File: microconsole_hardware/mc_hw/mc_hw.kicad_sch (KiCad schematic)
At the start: 39 parts, among them SW1 DPAD - UP, SW10 START, SW11 L1, SW12 R1, SW13 L2, SW14 R2, SW16 Joystick, SW17 Joystick, SW2 DPAD - DOWN, SW3 DPAD - LEFT, SW4 DPAD - RIGHT, SW5 A, SW6 B, SW7 X, SW8 Y, SW9 SELECT, U1 ILI9341 / ST7796S SPI LCD, U2 MAX98357A, U3 MCP23017x-x-SO

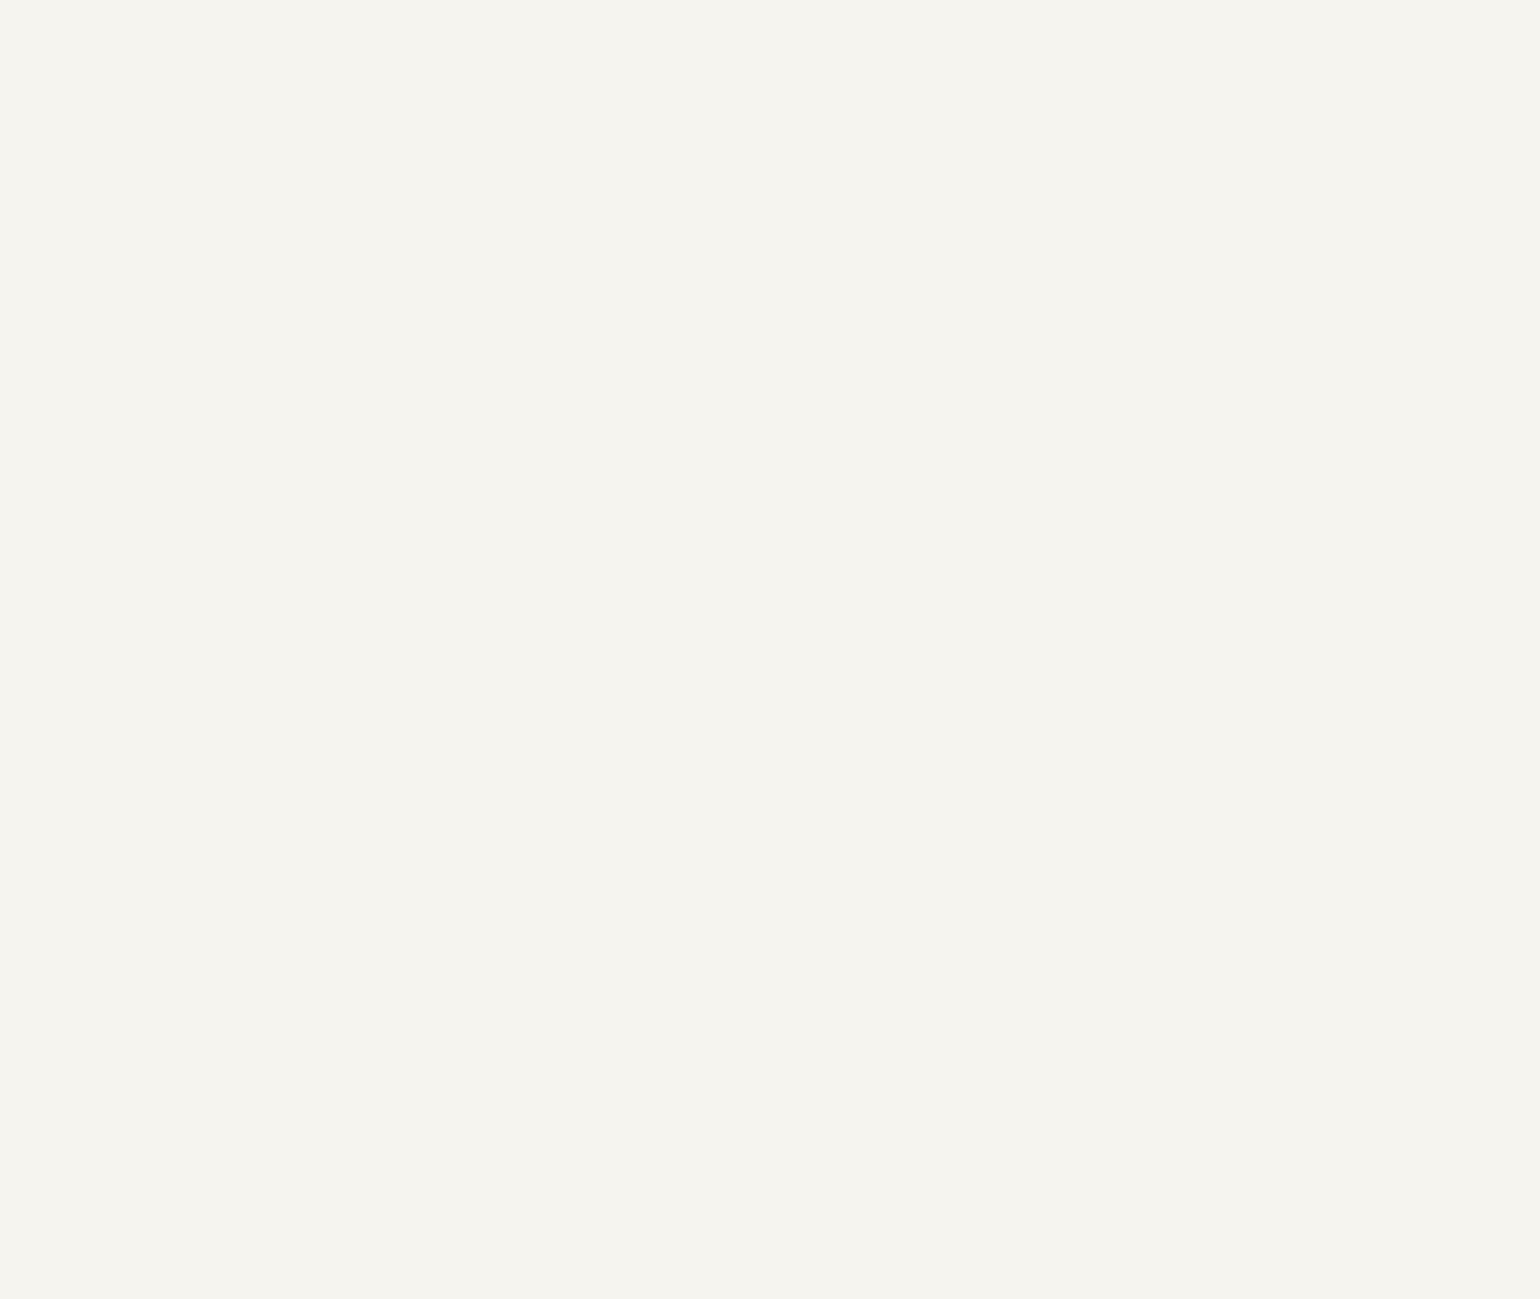
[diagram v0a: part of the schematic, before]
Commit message: hardware update
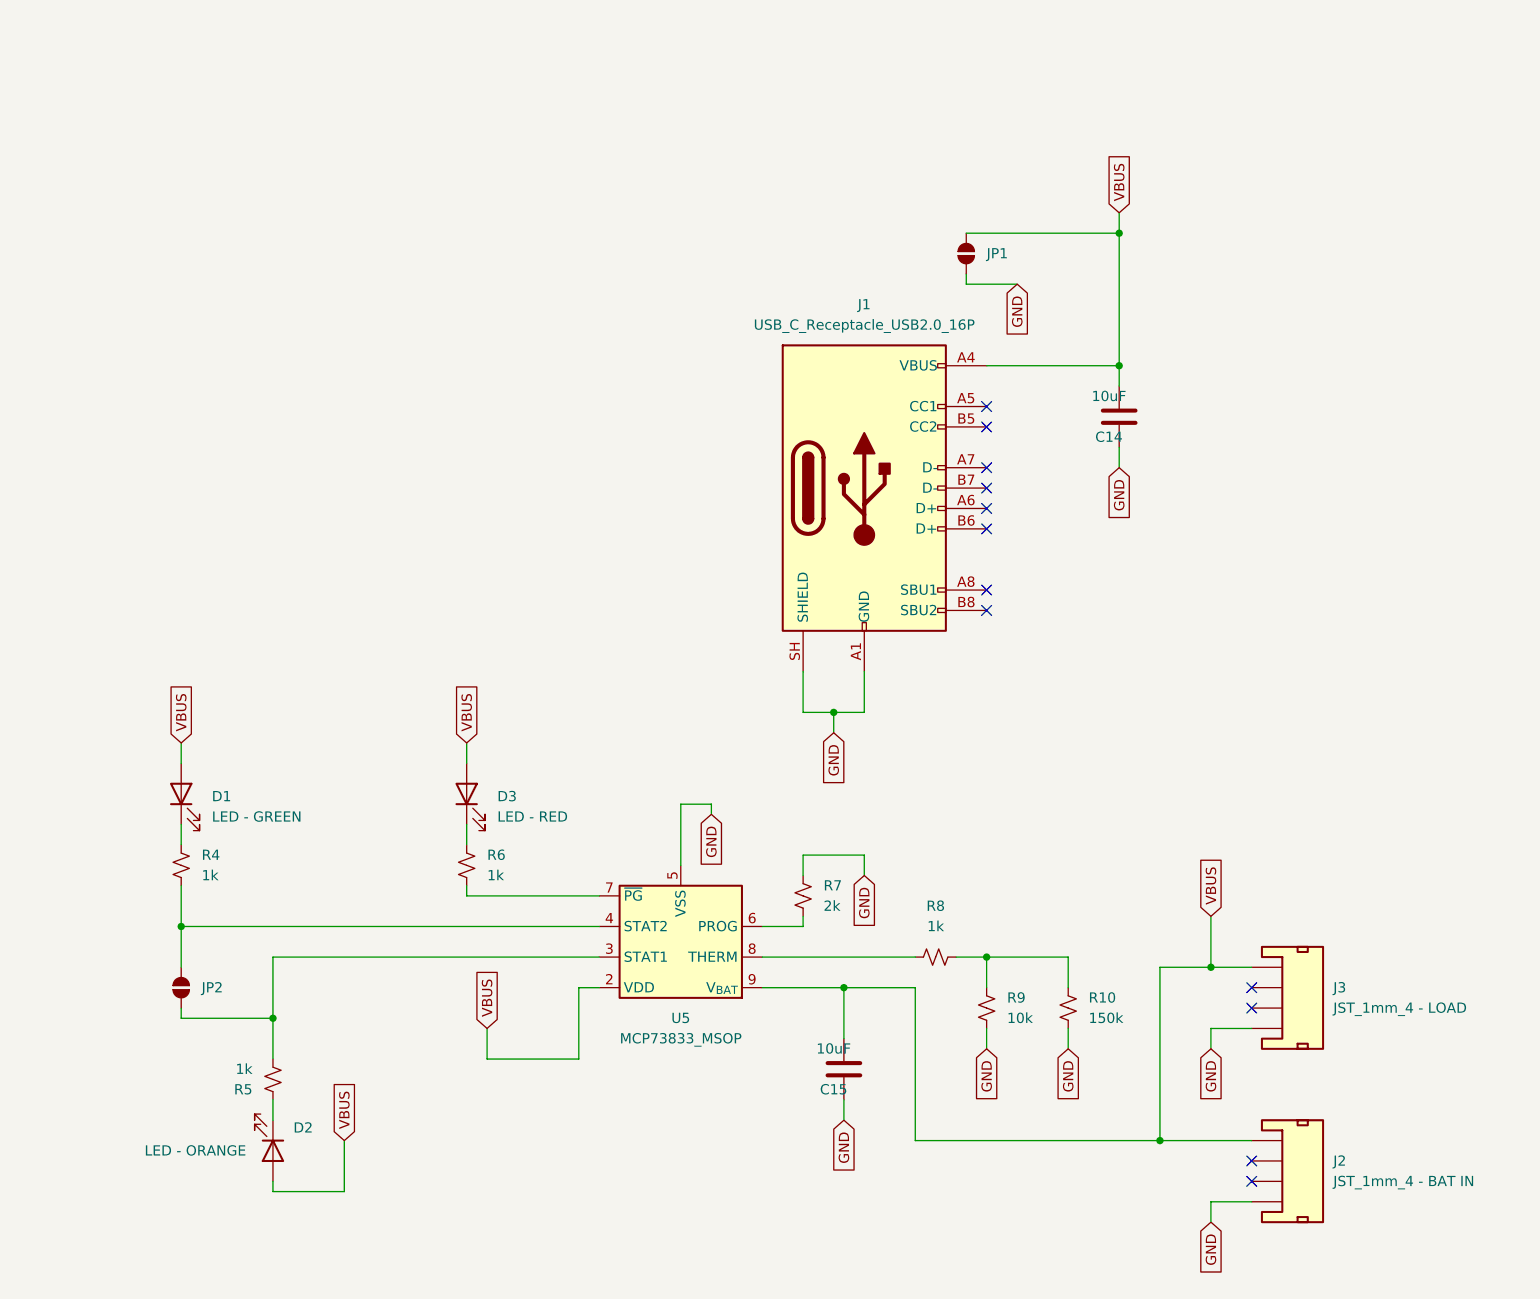
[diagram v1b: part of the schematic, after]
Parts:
- added C14, C15: 10uF, symbol Device:C
- added D1: LED - GREEN, PCM_SparkFun-Resistor:R_0603_1608Metric, symbol Device:LED
- added D2: LED - ORANGE, PCM_SparkFun-Resistor:R_0603_1608Metric, symbol Device:LED
- added D3: LED - RED, PCM_SparkFun-Resistor:R_0603_1608Metric, symbol Device:LED
- added J1: USB_C_Receptacle_USB2.0_16P, symbol Connector:USB_C_Receptacle_USB2.0_16P
- added J2: JST_1mm_4 - BAT IN, PCM_SparkFun-Connector:JST_1x04_P1.0mm_Horizontal_SMD, symbol PCM_SparkFun-Connector:Conn_01x04_JST_P1.0mm_Horizontal_SMD
- added J3: JST_1mm_4 - LOAD, PCM_SparkFun-Connector:JST_1x04_P1.0mm_Horizontal_SMD, symbol PCM_SparkFun-Connector:Conn_01x04_JST_P1.0mm_Horizontal_SMD
- added JP1, JP2: (no value), PCM_SparkFun-Jumper:Jumper_2_NO, symbol PCM_SparkFun-Jumper:SolderJumper_2_Open
- added R10: 150k, PCM_SparkFun-Resistor:R_0603_1608Metric, symbol PCM_SparkFun-Resistor:0.47_0603
- added R4, R5, R6, R8: 1k, PCM_SparkFun-Resistor:R_0603_1608Metric, symbol PCM_SparkFun-Resistor:0.47_0603
- added R7: 2k, PCM_SparkFun-Resistor:R_0603_1608Metric, symbol PCM_SparkFun-Resistor:0.47_0603
- added R9: 10k, PCM_SparkFun-Resistor:R_0603_1608Metric, symbol PCM_SparkFun-Resistor:0.47_0603
- added U5: MCP73833_MSOP, PCM_SparkFun-Semiconductor-Standard:MSOP-10_3x3mm_P0.5mm, symbol PCM_SparkFun-IC-Power:MCP73833
- SW16, SW17: footprint PCM_SparkFun-Switch:Joystick_PTH -> microconsole:Joystick_PTH
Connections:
- net GND: now also C14.1, C15.1, J1.A1 (GND), J1.A12 (GND), J1.B1 (GND), J1.B12 (GND), J1.SH (SHIELD), J2.4, J3.4, JP1.2 (B), R10.2, R7.2, R9.2, U5.5 (VSS)
- net VBUS renamed VDD
- net VDD: now also C14.2, C15.2, D1.2 (A), D2.2 (A), D3.2 (A), J1.A4 (VBUS), J1.A9 (VBUS), J1.B4 (VBUS), J1.B9 (VBUS), J2.1, J3.1, JP1.1 (A), U5.1 (VDD), U5.10 (V_{BAT}), U5.2 (VDD), U5.9 (V_{BAT})
- new net: R10.1, R8.1, R9.1
- new net: R8.2, U5.8 (THERM)
- new net: D1.1 (K), R4.2
- new net: D3.1 (K), R6.2
- new net: JP2.1 (A), R4.1, U5.4 (STAT2)
- new net: JP2.2 (B), R5.1, U5.3 (STAT1)
- new net: R6.1, U5.7 (~{PG})
- new net: D2.1 (K), R5.2
- new net: R7.1, U5.6 (PROG)
- no-connect marks 28 -> 40
